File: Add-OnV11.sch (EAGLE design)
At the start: 9 parts

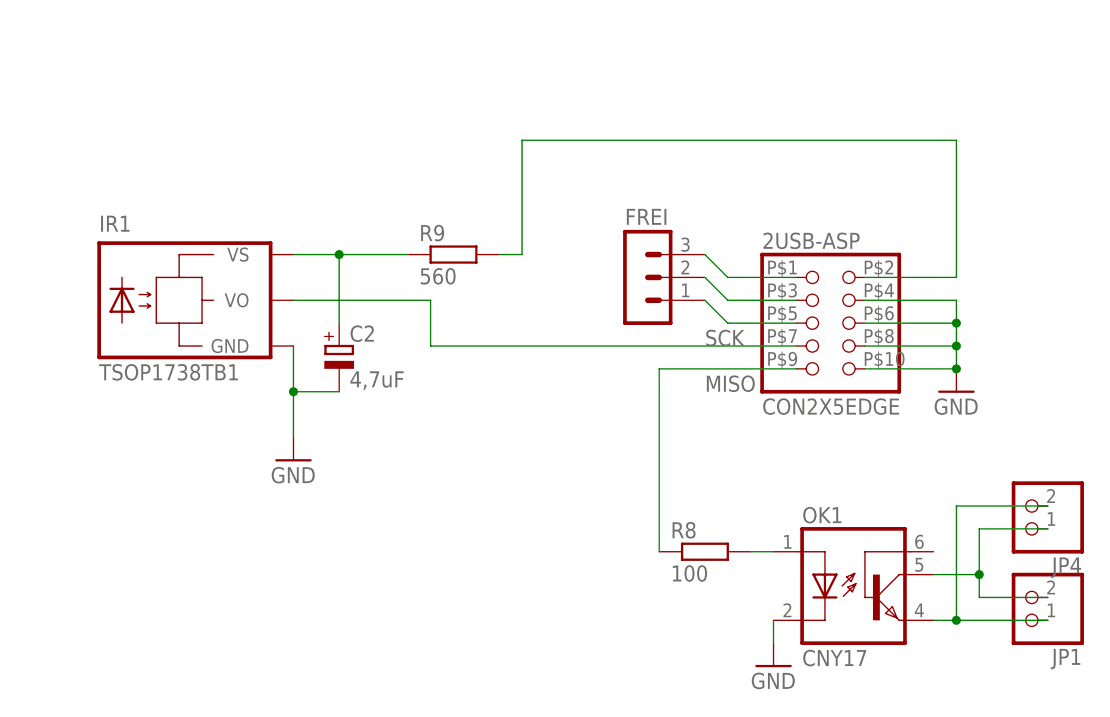
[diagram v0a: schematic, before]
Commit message: Optimized
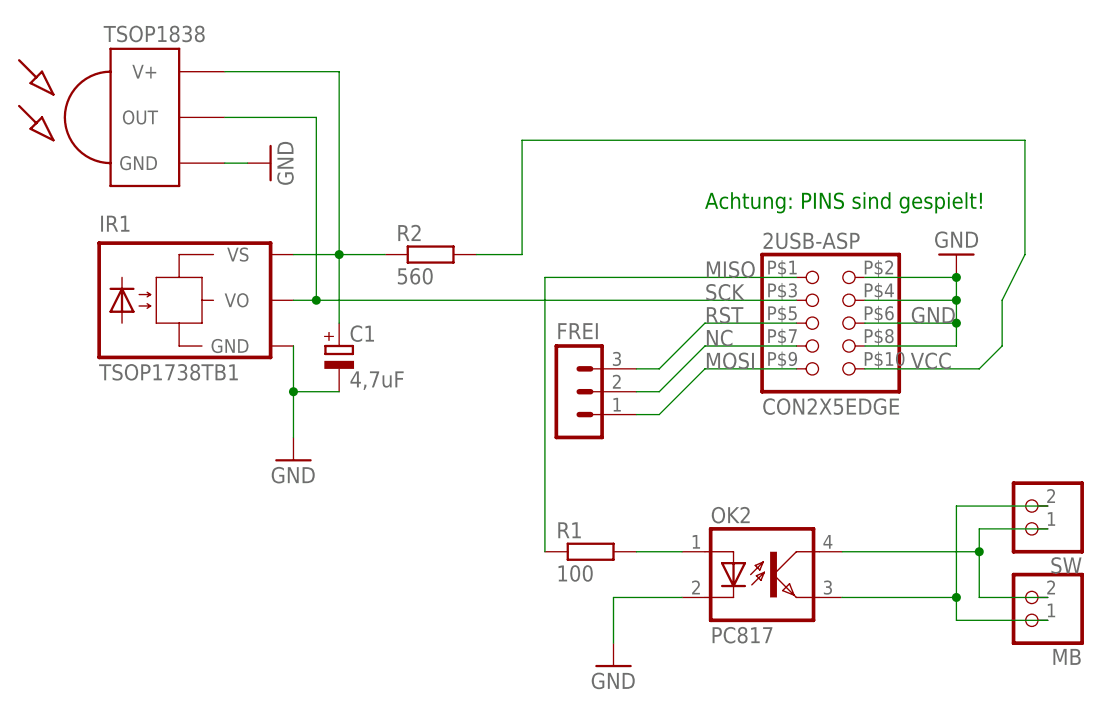
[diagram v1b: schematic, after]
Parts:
- removed OK1: CNY17, optocoupler:CNY17
- removed R8: 100, rcl:R-EU_0204/7
- removed R9: 560, rcl:R-EU_0204/7
- added OK2: PC817, optocoupler:PC817
- added R1: 100, rcl:R-EU_0204/2V
- added R2: 560, rcl:R-EU_0204/2V
- added U$1: TSOP1838, tsop-1:TSOP1838
- renumbered C2 to C1, JP1 to MB, JP4 to SW
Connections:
- removed net N$5: 2USB-ASP.2, R9.2
- removed net N$6: 2USB-ASP.5, FREI.1
- removed net N$7: 2USB-ASP.3, FREI.2
- removed net N$8: 2USB-ASP.1, FREI.3
- new net MOSI: 2USB-ASP.9, FREI.1
- new net NC: 2USB-ASP.7, FREI.2
- new net RST: 2USB-ASP.5, FREI.3
- new net VCC: 2USB-ASP.10, R2.2
- net GND: now also 2USB-ASP.2, OK2.C, U$1.GND; no longer 2USB-ASP.10, OK1.C
- net MISO: now also 2USB-ASP.1, R1.1; no longer 2USB-ASP.9, R8.1
- net N$1: now also R2.1, U$1.V+; no longer R9.1
- net N$2: now also OK2.A, R1.2; no longer OK1.A, R8.2
- net N$3: now also OK2.COL; no longer OK1.COL
- net N$4: now also OK2.EMIT; no longer OK1.EMI
- net SCK: now also 2USB-ASP.3, U$1.OUT; no longer 2USB-ASP.7
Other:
- note added: "Achtung: PINS sind gespielt!"
- moved on the sheet: FREI
